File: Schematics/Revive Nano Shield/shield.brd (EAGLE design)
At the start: 35.6 x 63.5 mm, 24 parts

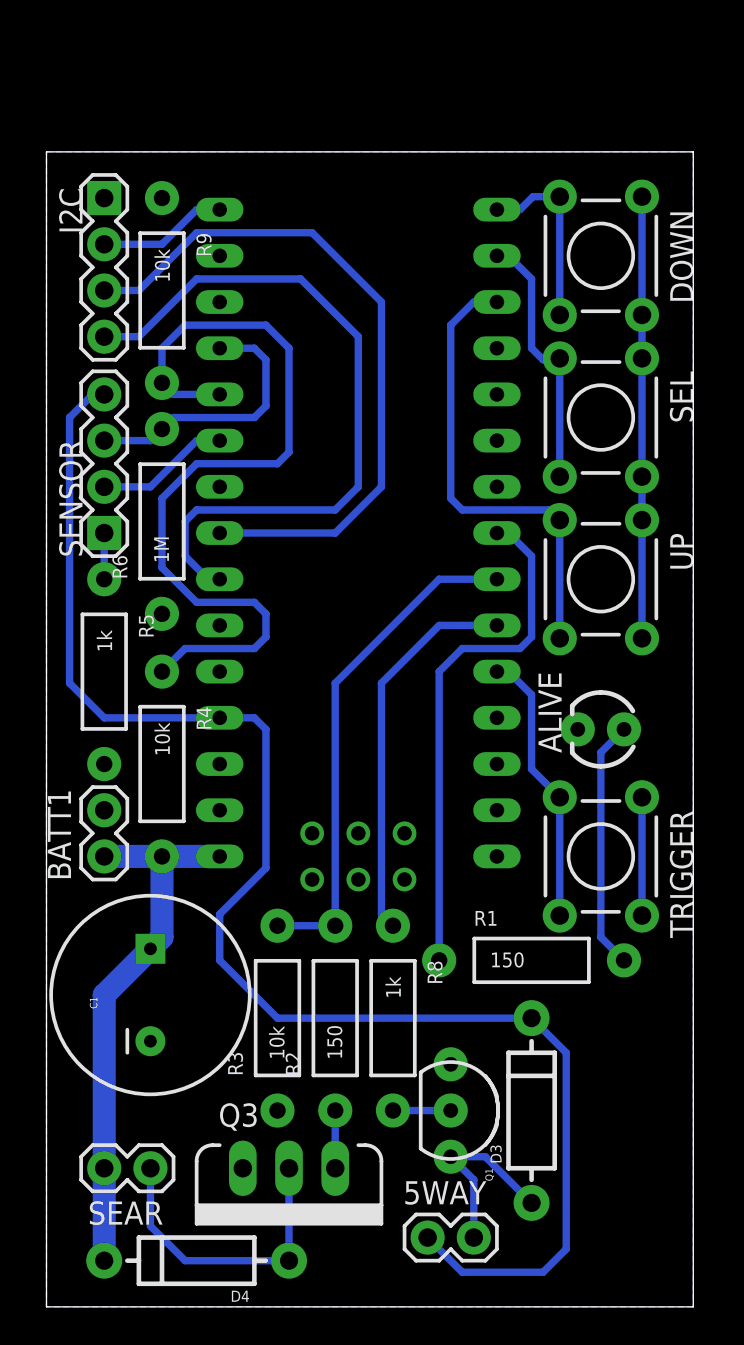
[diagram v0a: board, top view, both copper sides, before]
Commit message: Updated schematics
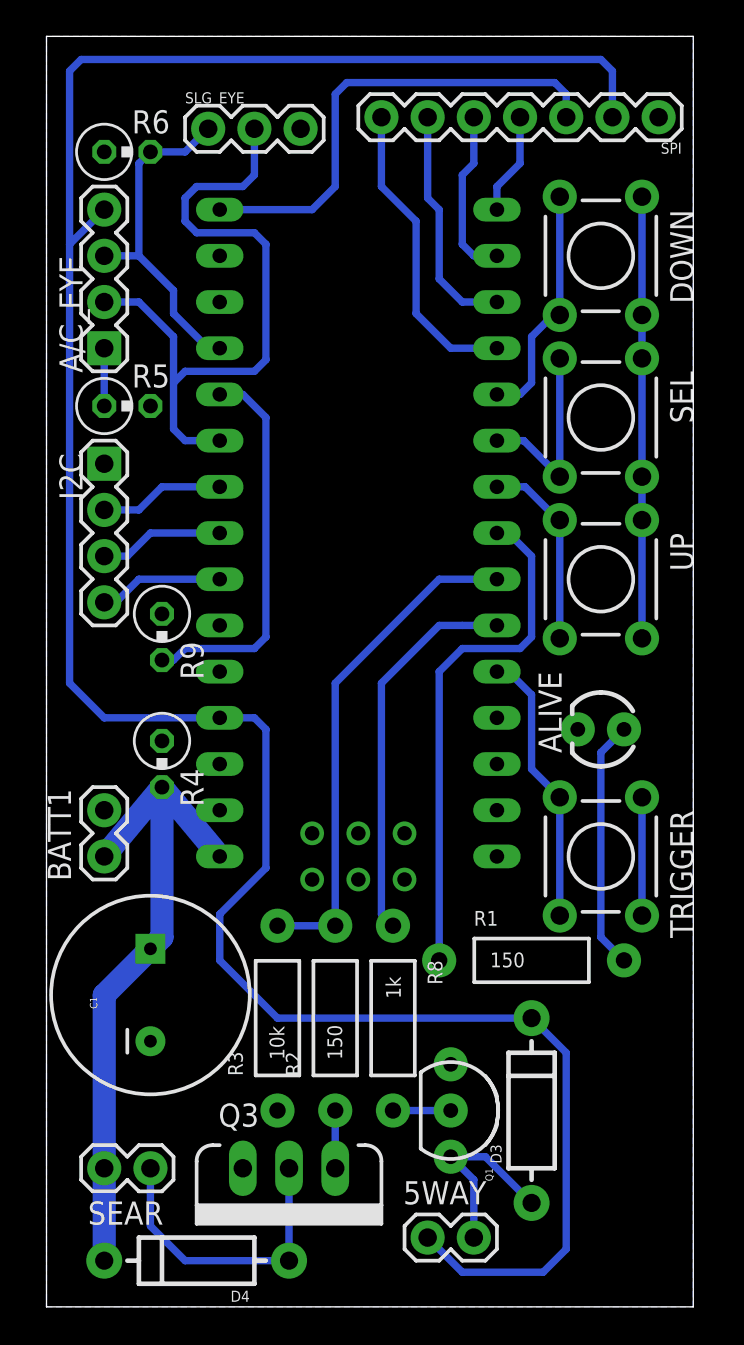
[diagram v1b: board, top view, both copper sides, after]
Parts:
- removed SENSOR: (no value), SparkFun:1X04
- added A/C_EYE: (no value), SparkFun:1X04
- added SLG_EYE: (no value), SparkFun-Connectors:1X03
- added SPI: (no value), SparkFun-Connectors:1X07
- R4, R5, R6, R9: device SparkFun:AXIAL-0.4 -> resistor:0309V
- moved R6 20.4 mm to (4.45, 63.5), turned to 0 degrees
- moved R9 19.1 mm to (6.35, 36.8)
- moved R5 14.7 mm to (4.45, 49.5), turned to 0 degrees
- moved I2C 14.6 mm to (3.17, 46.4)
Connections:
- net SCL renamed I2C_CLK
- net SDA renamed I2C_SDA
- removed net IRED: SENSOR.2, U$5.A2
- removed net N$6: R5.P$1, SENSOR.1
- removed net SENSOR: R6.P$2, SENSOR.3, U$5.A0
- new net EYE_GND: A/C_EYE.1, R5.1
- new net EYE_PWR: A/C_EYE.2, SLG_EYE.2, U$5.A2
- new net EYE_READ: A/C_EYE.3, R6.2, SLG_EYE.1, U$5.A0
- new net N$12: U$5.TX0
- new net N$13: U$5.RX1
- new net SPI_CLK: SPI.3, U$5.D13
- new net SPI_CS: SPI.7, U$5.D9
- new net SPI_DC: SPI.6, U$5.D10
- new net SPI_MOSI: SPI.5, U$5.D11
- new net SPI_RES: SPI.4, U$5.D12
- net 5V: now also A/C_EYE.4, SPI.2; no longer SENSOR.4
- net 9V: now also R4.2; no longer R4.P$2
- net BATT_STATUS: now also R4.1, R9.2; no longer R4.P$1, R9.P$2
- net DWN_BTN: now also U$5.D8; no longer U$5.D12
- net GND: now also R5.2, R6.1, R9.1, SLG_EYE.3, SPI.1; no longer R5.P$2, R6.P$1, R9.P$1
- net OLED_PWR: now also U$5.A3; no longer U$5.D13
- net SEL_BTN: now also U$5.D7; no longer U$5.D11
- net UP_BTN: now also U$5.D6; no longer U$5.D10
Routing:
- net 5V: track 83.5 -> 135.7 mm
- net EYE_PWR: track 0.00 -> 37.6 mm
- net I2C_CLK: track 39.5 -> 6.88 mm
- net I2C_SDA: track 38.2 -> 6.88 mm
- net SPI_CLK: track 0.00 -> 27.1 mm
- net BATT_STATUS: track 45.5 -> 21.4 mm
- net EYE_READ: track 0.00 -> 18.9 mm
- net SPI_CS: track 0.00 -> 16.8 mm
- net SENSOR: track 15.0 -> 0.00 mm
- net UP_BTN: track 25.6 -> 10.7 mm
- net SPI_DC: track 0.00 -> 12.9 mm
- net SPI_MOSI: track 0.00 -> 9.42 mm
- net IRED: track 7.40 -> 0.00 mm
- net 9V: track 29.9 -> 37.3 mm
- net SPI_RES: track 0.00 -> 5.61 mm
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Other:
- board size 35.6 x 63.5 mm -> 35.6 x 69.8 mm
